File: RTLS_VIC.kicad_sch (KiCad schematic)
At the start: 41 parts, among them J10 Conn_01x04_Socket, J11 Conn_01x04_Socket, J12 Conn_01x02_Pin, J13 Conn_01x04_Socket, J14 Conn_01x03_Pin, J15 Conn_01x03_Pin, J16 Conn_01x03_Pin, J17 Conn_01x03_Pin, J8 Conn_01x02_Pin, SW1 TS-1187A-B-A-B, U2 TPS63900DSKR, U9 STM32F411RET6, X1 XL2EL89COI-111YLC-26M

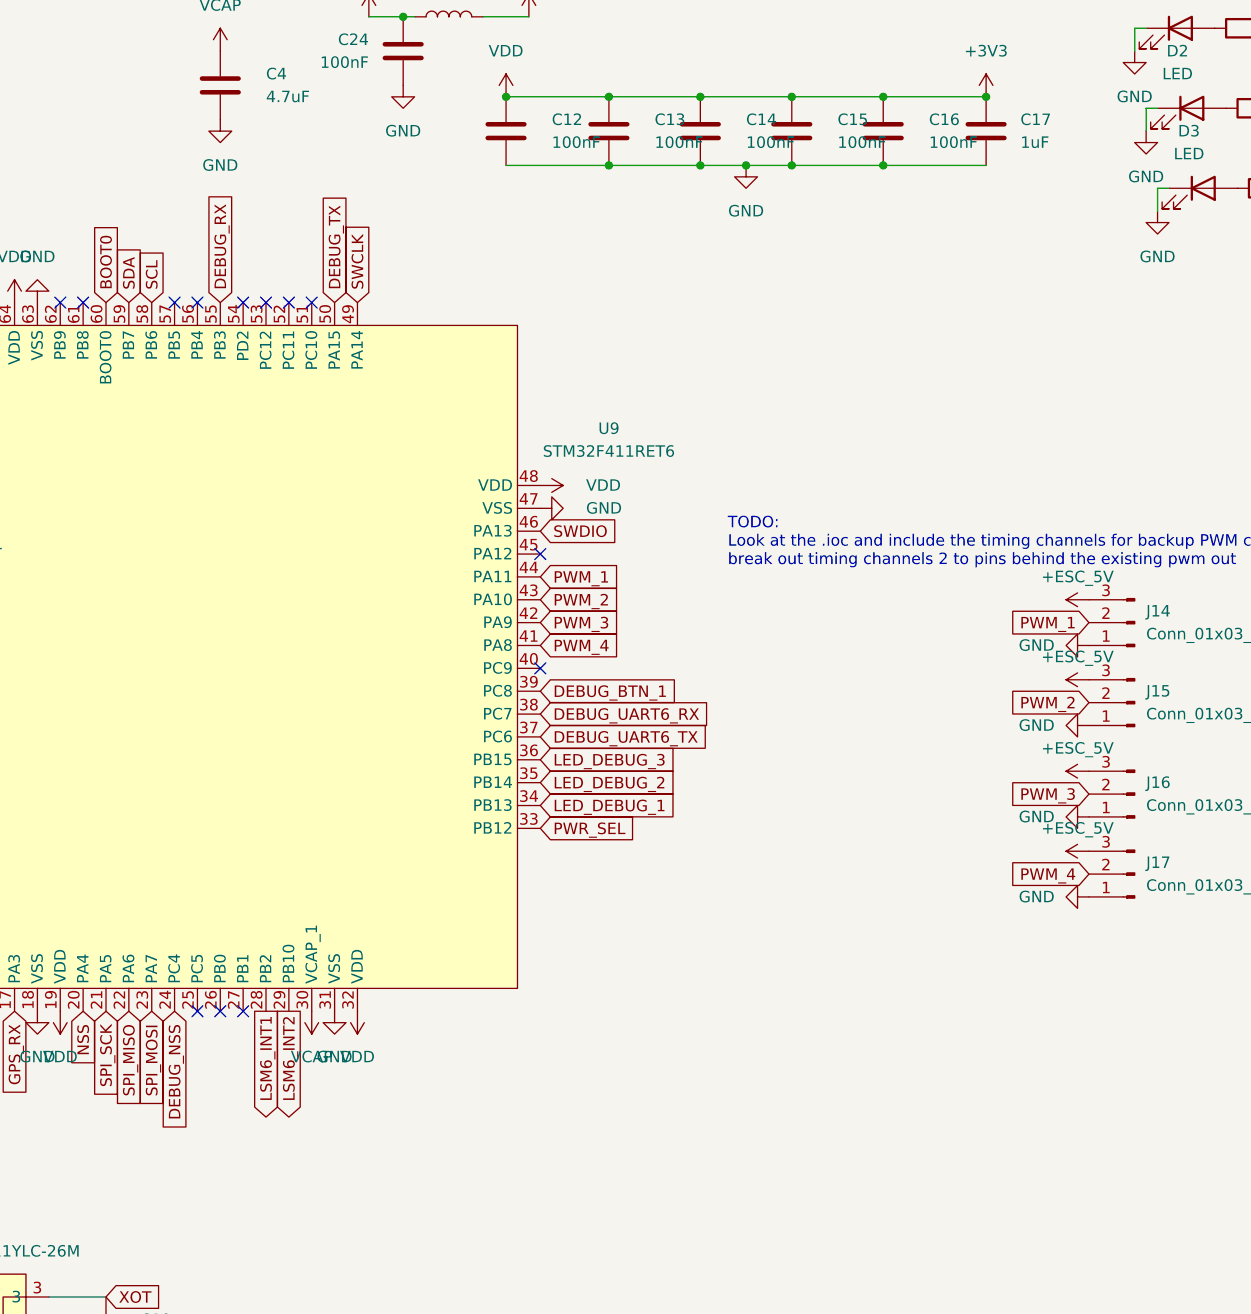
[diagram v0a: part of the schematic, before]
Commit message: sponsor and timing
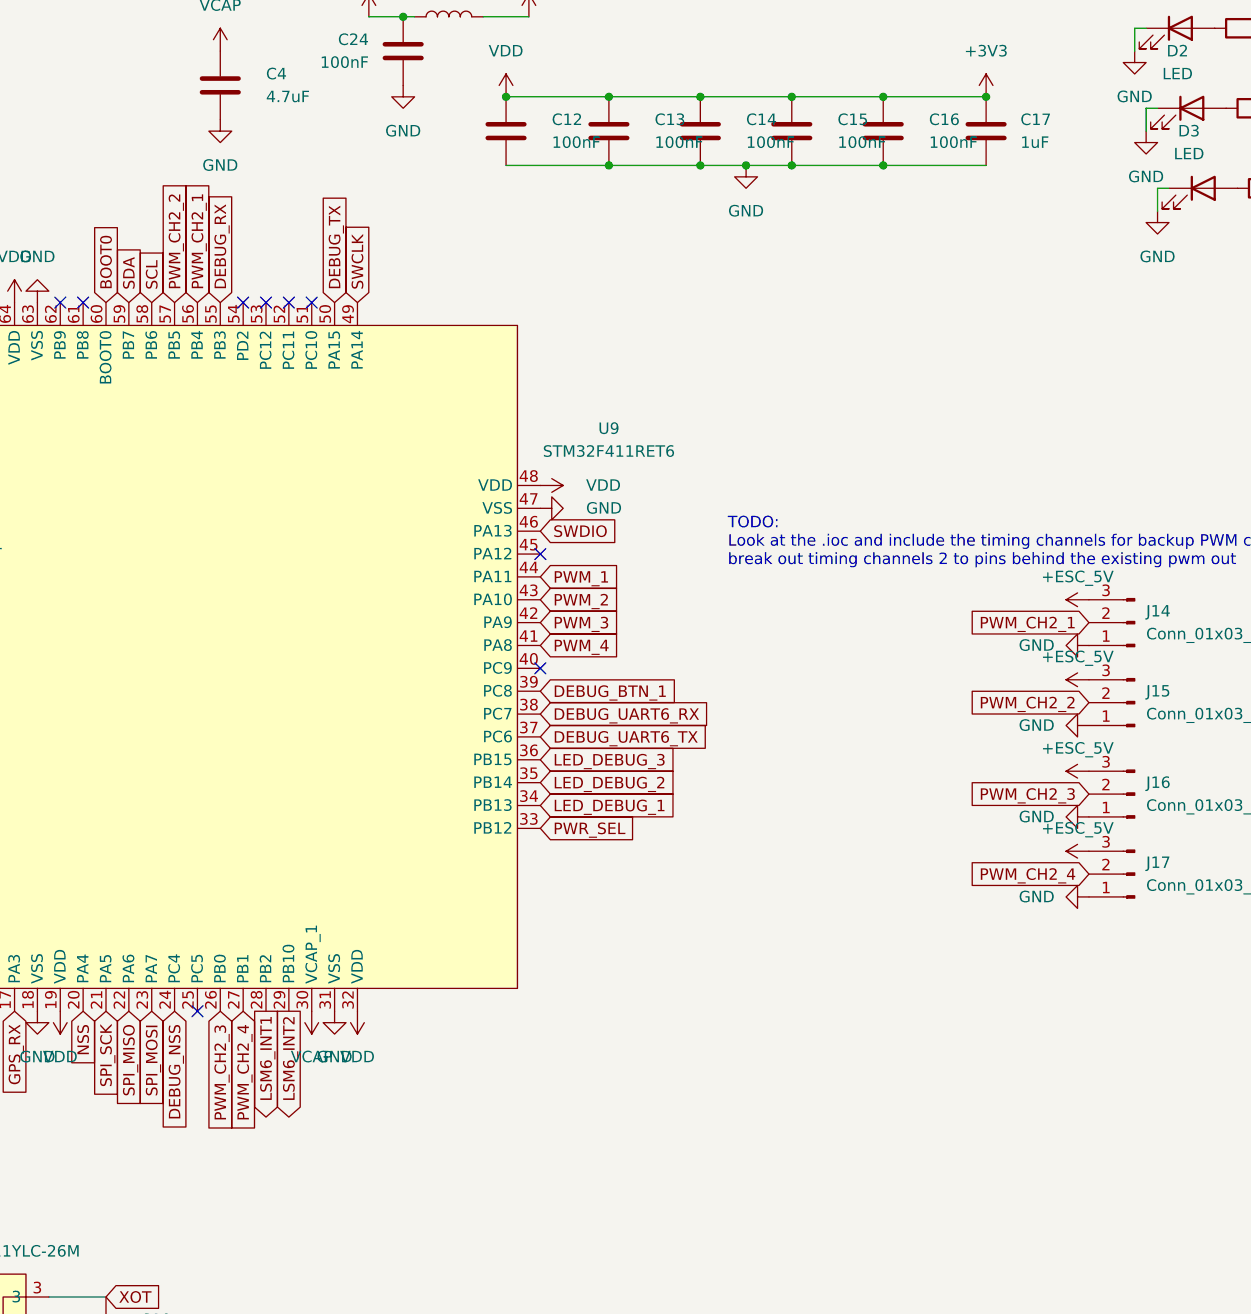
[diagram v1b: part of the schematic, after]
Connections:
- net PWM_1: no longer J14.2 (Pin_2)
- net PWM_2: no longer J15.2 (Pin_2)
- net PWM_3: no longer J16.2 (Pin_2)
- net PWM_4: no longer J17.2 (Pin_2)
- net PWM_CH2_3: now reaches U9.26 (PB0)
- net PWM_CH2_3: now also J16.2 (Pin_2)
- net PWM_CH2_4: now reaches U9.27 (PB1)
- net PWM_CH2_4: now also J17.2 (Pin_2)
- net PWM_CH2_1: now reaches U9.56 (PB4)
- net PWM_CH2_1: now also J14.2 (Pin_2)
- net PWM_CH2_2: now reaches U9.57 (PB5)
- net PWM_CH2_2: now also J15.2 (Pin_2)
- no-connect marks 24 -> 20
